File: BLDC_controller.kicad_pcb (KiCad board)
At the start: 4 copper layers, 50 x 35 mm, 95 parts, among them P2 CONN_01X06, P3 CONN_01X05, P5 CONN_01X05, Q1 PSMN2R0-30YLD, Q2 PSMN2R0-30YLD, Q3 PSMN2R0-30YLD, Q4 PSMN2R0-30YLD, Q5 PSMN2R0-30YLD, Q6 PSMN2R0-30YLD

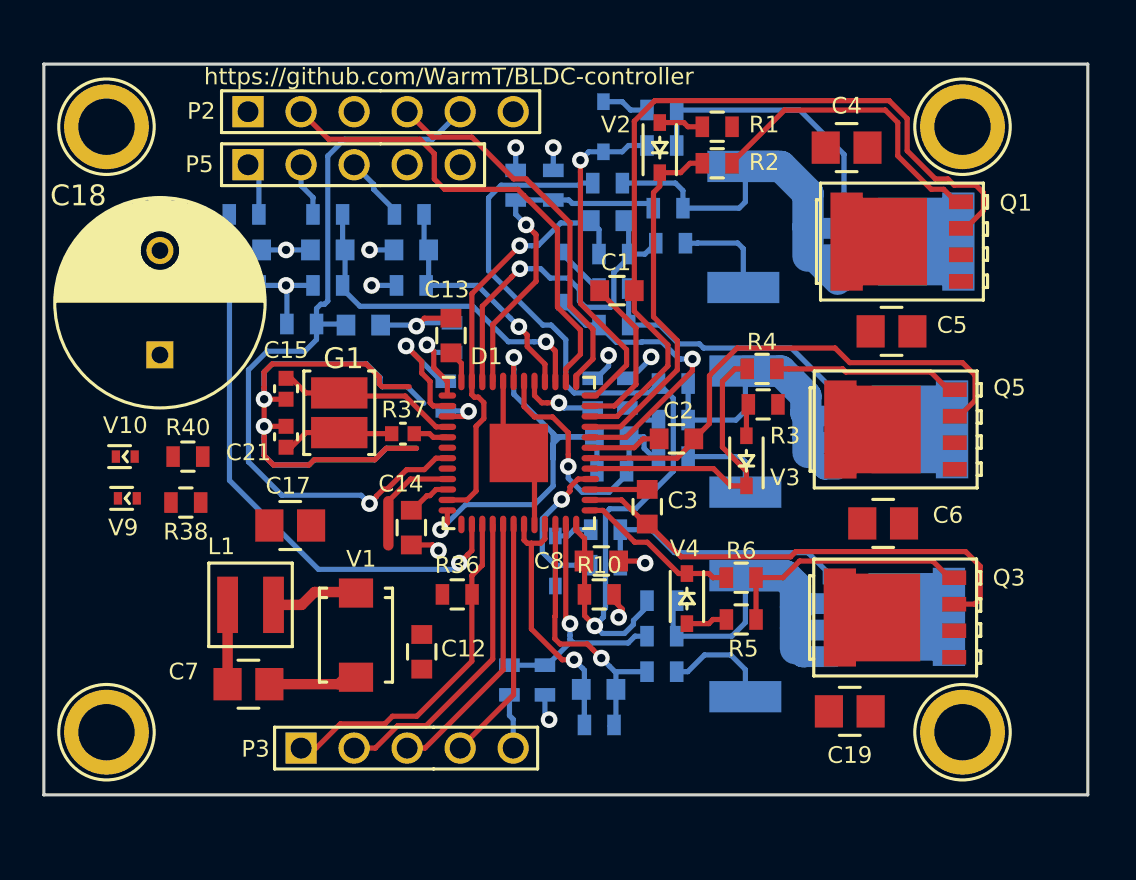
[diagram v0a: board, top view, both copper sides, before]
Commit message: Layout ready for 1st review
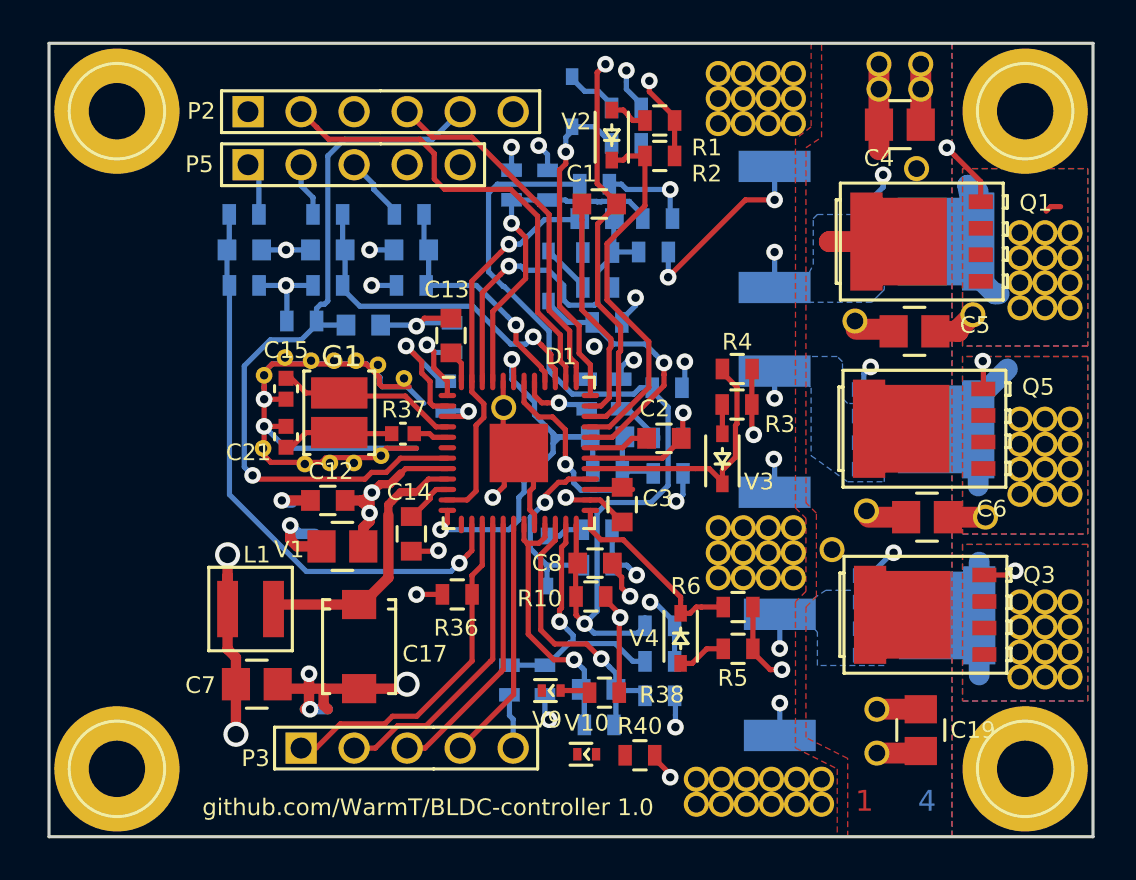
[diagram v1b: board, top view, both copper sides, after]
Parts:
- removed C18: 680u, project_footprints:C_Radial_D10_L25_P5
- added REF**: VIA-0.8mm-0.4mm, project_footprints:VIA-0.8mm-0.4mm, F.Cu at (151.2, 97.8)
- added REF**: VIA-0.8mm-0.4mm, project_footprints:VIA-0.8mm-0.4mm, F.Cu at (149.9, 93.2)
- added REF**: VIA-1.2mm-0.8mm, project_footprints:VIA-1.2mm-0.8mm, F.Cu at (166.2, 113.2)
- added REF**: VIA-0.8mm-0.4mm, project_footprints:VIA-0.8mm-0.4mm, F.Cu at (147.8, 93.2)
- added REF**: VIA-0.8mm-0.4mm, project_footprints:VIA-0.8mm-0.4mm, F.Cu at (148.9, 93.2)
- added REF**: VIA-1.2mm-0.8mm, project_footprints:VIA-1.2mm-0.8mm, F.Cu at (172.8, 102.3)
- added REF**: VIA-1.2mm-0.8mm, project_footprints:VIA-1.2mm-0.8mm, F.Cu at (180.1, 100.7)
- added REF**: VIA-1.2mm-0.8mm, project_footprints:VIA-1.2mm-0.8mm, F.Cu at (174.9, 112.0)
- added REF**: VIA-1.2mm-0.8mm, project_footprints:VIA-1.2mm-0.8mm, F.Cu at (174.9, 109.9)
- added REF**: VIA-1.2mm-0.8mm, project_footprints:VIA-1.2mm-0.8mm, F.Cu at (174.4, 100.4)
- added REF**: VIA-1.2mm-0.8mm, project_footprints:VIA-1.2mm-0.8mm, F.Cu at (173.8, 91.3)
- added REF**: VIA-1.2mm-0.8mm, project_footprints:VIA-1.2mm-0.8mm, F.Cu at (179.5, 91.0)
- added REF**: VIA-1.2mm-0.8mm, project_footprints:VIA-1.2mm-0.8mm, F.Cu at (176.8, 84.0)
- added REF**: VIA-0.8mm-0.4mm, project_footprints:VIA-0.8mm-0.4mm, F.Cu at (149.8, 98.1)
- added REF**: VIA-1.2mm-0.8mm, project_footprints:VIA-1.2mm-0.8mm, F.Cu at (177.0, 79.0)
- added REF**: VIA-1.2mm-0.8mm, project_footprints:VIA-1.2mm-0.8mm, F.Cu at (177.0, 80.2)
- added REF**: VIA-1.2mm-0.8mm, project_footprints:VIA-1.2mm-0.8mm, F.Cu at (175.0, 80.2)
- added REF**: VIA-1.2mm-0.8mm, project_footprints:VIA-1.2mm-0.8mm, F.Cu at (175.0, 79.0)
- added REF**: VIA-1.2mm-0.8mm, project_footprints:VIA-1.2mm-0.8mm, F.Cu at (170.9, 81.8)
- added REF**: VIA-1.2mm-0.8mm, project_footprints:VIA-1.2mm-0.8mm, F.Cu at (169.7, 81.8)
- added REF**: VIA-1.2mm-0.8mm, project_footprints:VIA-1.2mm-0.8mm, F.Cu at (168.5, 81.8)
- added REF**: VIA-1.2mm-0.8mm, project_footprints:VIA-1.2mm-0.8mm, F.Cu at (167.3, 81.8)
- added REF**: VIA-1.2mm-0.8mm, project_footprints:VIA-1.2mm-0.8mm, F.Cu at (170.9, 80.7)
- added REF**: VIA-1.2mm-0.8mm, project_footprints:VIA-1.2mm-0.8mm, F.Cu at (169.7, 80.7)
- added REF**: VIA-0.8mm-0.4mm, project_footprints:VIA-0.8mm-0.4mm, F.Cu at (148.7, 98.1)
- added REF**: VIA-1.2mm-0.8mm, project_footprints:VIA-1.2mm-0.8mm, F.Cu at (168.5, 80.7)
- added REF**: VIA-1.2mm-0.8mm, project_footprints:VIA-1.2mm-0.8mm, F.Cu at (167.3, 80.7)
- added REF**: VIA-1.2mm-0.8mm, project_footprints:VIA-1.2mm-0.8mm, F.Cu at (170.9, 79.5)
- added REF**: VIA-1.2mm-0.8mm, project_footprints:VIA-1.2mm-0.8mm, F.Cu at (169.7, 79.5)
- added REF**: VIA-1.2mm-0.8mm, project_footprints:VIA-1.2mm-0.8mm, F.Cu at (168.5, 79.5)
- added REF**: VIA-1.2mm-0.8mm, project_footprints:VIA-1.2mm-0.8mm, F.Cu at (169.7, 103.6)
- added REF**: VIA-1.2mm-0.8mm, project_footprints:VIA-1.2mm-0.8mm, F.Cu at (168.5, 103.6)
- added REF**: VIA-1.2mm-0.8mm, project_footprints:VIA-1.2mm-0.8mm, F.Cu at (167.3, 103.6)
- added REF**: VIA-1.2mm-0.8mm, project_footprints:VIA-1.2mm-0.8mm, F.Cu at (170.9, 103.6)
- added REF**: VIA-1.2mm-0.8mm, project_footprints:VIA-1.2mm-0.8mm, F.Cu at (169.7, 102.4)
- added REF**: VIA-0.8mm-0.4mm, project_footprints:VIA-0.8mm-0.4mm, F.Cu at (146.6, 93.1)
- added REF**: VIA-1.2mm-0.8mm, project_footprints:VIA-1.2mm-0.8mm, F.Cu at (168.5, 102.4)
- added REF**: VIA-1.2mm-0.8mm, project_footprints:VIA-1.2mm-0.8mm, F.Cu at (167.3, 102.4)
- added REF**: VIA-1.2mm-0.8mm, project_footprints:VIA-1.2mm-0.8mm, F.Cu at (170.9, 102.4)
- added REF**: VIA-1.2mm-0.8mm, project_footprints:VIA-1.2mm-0.8mm, F.Cu at (169.7, 101.2)
- added REF**: VIA-1.2mm-0.8mm, project_footprints:VIA-1.2mm-0.8mm, F.Cu at (168.5, 101.2)
- added REF**: VIA-1.2mm-0.8mm, project_footprints:VIA-1.2mm-0.8mm, F.Cu at (167.3, 101.2)
- added REF**: VIA-1.2mm-0.8mm, project_footprints:VIA-1.2mm-0.8mm, F.Cu at (170.9, 101.2)
- added REF**: VIA-1.2mm-0.8mm, project_footprints:VIA-1.2mm-0.8mm, F.Cu at (184.2, 108.4)
- added REF**: VIA-1.2mm-0.8mm, project_footprints:VIA-1.2mm-0.8mm, F.Cu at (182.9, 108.4)
- added REF**: VIA-1.2mm-0.8mm, project_footprints:VIA-1.2mm-0.8mm, F.Cu at (181.8, 108.4)
- added REF**: VIA-0.8mm-0.4mm, project_footprints:VIA-0.8mm-0.4mm, F.Cu at (147.5, 98.2)
- added REF**: VIA-1.2mm-0.8mm, project_footprints:VIA-1.2mm-0.8mm, F.Cu at (184.2, 107.2)
- added REF**: VIA-1.2mm-0.8mm, project_footprints:VIA-1.2mm-0.8mm, F.Cu at (182.9, 107.2)
- added REF**: VIA-1.2mm-0.8mm, project_footprints:VIA-1.2mm-0.8mm, F.Cu at (181.8, 107.2)
- added REF**: VIA-1.2mm-0.8mm, project_footprints:VIA-1.2mm-0.8mm, F.Cu at (184.2, 106.0)
- added REF**: VIA-1.2mm-0.8mm, project_footprints:VIA-1.2mm-0.8mm, F.Cu at (182.9, 106.0)
- added REF**: VIA-1.2mm-0.8mm, project_footprints:VIA-1.2mm-0.8mm, F.Cu at (181.8, 106.0)
- added REF**: VIA-1.2mm-0.8mm, project_footprints:VIA-1.2mm-0.8mm, F.Cu at (184.2, 104.8)
- added REF**: VIA-1.2mm-0.8mm, project_footprints:VIA-1.2mm-0.8mm, F.Cu at (182.9, 104.8)
- added REF**: VIA-1.2mm-0.8mm, project_footprints:VIA-1.2mm-0.8mm, F.Cu at (181.8, 104.8)
- added REF**: VIA-1.2mm-0.8mm, project_footprints:VIA-1.2mm-0.8mm, F.Cu at (184.2, 99.6)
- added REF**: VIA-0.8mm-0.4mm, project_footprints:VIA-0.8mm-0.4mm, F.Cu at (145.5, 97.4)
- added REF**: VIA-1.2mm-0.8mm, project_footprints:VIA-1.2mm-0.8mm, F.Cu at (182.9, 99.6)
- added REF**: VIA-1.2mm-0.8mm, project_footprints:VIA-1.2mm-0.8mm, F.Cu at (181.8, 99.6)
- added REF**: VIA-1.2mm-0.8mm, project_footprints:VIA-1.2mm-0.8mm, F.Cu at (184.2, 98.4)
- added REF**: VIA-1.2mm-0.8mm, project_footprints:VIA-1.2mm-0.8mm, F.Cu at (182.9, 98.4)
- added REF**: VIA-1.2mm-0.8mm, project_footprints:VIA-1.2mm-0.8mm, F.Cu at (181.8, 98.4)
- added REF**: VIA-1.2mm-0.8mm, project_footprints:VIA-1.2mm-0.8mm, F.Cu at (184.2, 97.2)
- added REF**: VIA-1.2mm-0.8mm, project_footprints:VIA-1.2mm-0.8mm, F.Cu at (182.9, 97.2)
- added REF**: VIA-1.2mm-0.8mm, project_footprints:VIA-1.2mm-0.8mm, F.Cu at (181.8, 97.2)
- added REF**: VIA-1.2mm-0.8mm, project_footprints:VIA-1.2mm-0.8mm, F.Cu at (184.2, 96.0)
- added REF**: VIA-1.2mm-0.8mm, project_footprints:VIA-1.2mm-0.8mm, F.Cu at (182.9, 96.0)
- added REF**: VIA-0.8mm-0.4mm, project_footprints:VIA-0.8mm-0.4mm, F.Cu at (145.6, 93.9)
- added REF**: VIA-1.2mm-0.8mm, project_footprints:VIA-1.2mm-0.8mm, F.Cu at (181.8, 96.0)
- added REF**: VIA-1.2mm-0.8mm, project_footprints:VIA-1.2mm-0.8mm, F.Cu at (184.2, 90.7)
- added REF**: VIA-1.2mm-0.8mm, project_footprints:VIA-1.2mm-0.8mm, F.Cu at (182.9, 90.7)
- added REF**: VIA-1.2mm-0.8mm, project_footprints:VIA-1.2mm-0.8mm, F.Cu at (181.8, 90.7)
- added REF**: VIA-1.2mm-0.8mm, project_footprints:VIA-1.2mm-0.8mm, F.Cu at (184.2, 89.5)
- added REF**: VIA-1.2mm-0.8mm, project_footprints:VIA-1.2mm-0.8mm, F.Cu at (182.9, 89.5)
- added REF**: VIA-1.2mm-0.8mm, project_footprints:VIA-1.2mm-0.8mm, F.Cu at (181.8, 89.5)
- added REF**: VIA-1.2mm-0.8mm, project_footprints:VIA-1.2mm-0.8mm, F.Cu at (184.2, 88.3)
- added REF**: VIA-1.2mm-0.8mm, project_footprints:VIA-1.2mm-0.8mm, F.Cu at (182.9, 88.3)
- added REF**: VIA-1.2mm-0.8mm, project_footprints:VIA-1.2mm-0.8mm, F.Cu at (181.8, 88.3)
- added REF**: VIA-0.8mm-0.4mm, project_footprints:VIA-0.8mm-0.4mm, F.Cu at (152.2, 94.1)
- added REF**: VIA-1.2mm-0.8mm, project_footprints:VIA-1.2mm-0.8mm, F.Cu at (184.2, 87.1)
- added REF**: VIA-1.2mm-0.8mm, project_footprints:VIA-1.2mm-0.8mm, F.Cu at (182.9, 87.1)
- added REF**: VIA-1.2mm-0.8mm, project_footprints:VIA-1.2mm-0.8mm, F.Cu at (181.8, 87.1)
- added REF**: VIA-1.2mm-0.8mm, project_footprints:VIA-1.2mm-0.8mm, F.Cu at (157.0, 95.5)
- added REF**: VIA-1.2mm-0.8mm, project_footprints:VIA-1.2mm-0.8mm, F.Cu at (172.2, 114.5)
- added REF**: VIA-1.2mm-0.8mm, project_footprints:VIA-1.2mm-0.8mm, F.Cu at (171.1, 114.5)
- added REF**: VIA-1.2mm-0.8mm, project_footprints:VIA-1.2mm-0.8mm, F.Cu at (169.8, 114.5)
- added REF**: VIA-1.2mm-0.8mm, project_footprints:VIA-1.2mm-0.8mm, F.Cu at (168.7, 114.5)
- added REF**: VIA-1.2mm-0.8mm, project_footprints:VIA-1.2mm-0.8mm, F.Cu at (167.4, 114.5)
- added REF**: VIA-0.8mm-0.4mm, project_footprints:VIA-0.8mm-0.4mm, F.Cu at (151.0, 93.4)
- added REF**: VIA-1.2mm-0.8mm, project_footprints:VIA-1.2mm-0.8mm, F.Cu at (166.2, 114.5)
- added REF**: VIA-1.2mm-0.8mm, project_footprints:VIA-1.2mm-0.8mm, F.Cu at (172.2, 113.2)
- added REF**: VIA-1.2mm-0.8mm, project_footprints:VIA-1.2mm-0.8mm, F.Cu at (171.1, 113.2)
- added REF**: VIA-1.2mm-0.8mm, project_footprints:VIA-1.2mm-0.8mm, F.Cu at (169.8, 113.2)
- added REF**: VIA-1.2mm-0.8mm, project_footprints:VIA-1.2mm-0.8mm, F.Cu at (168.7, 113.2)
- added REF**: VIA-1.2mm-0.8mm, project_footprints:VIA-1.2mm-0.8mm, F.Cu at (167.4, 113.2)
- added REF**: VIA-1.2mm-0.8mm, project_footprints:VIA-1.2mm-0.8mm, F.Cu at (167.3, 79.5)
- moved V10 26.3 mm to (161.0, 112.1)
- moved R40 25.9 mm to (163.6, 112.1)
- moved V9 22.3 mm to (159.3, 109.0)
- moved R38 22.0 mm to (161.8, 109.1)
- moved C12 8.53 mm to (148.6, 99.9), turned to 180 degrees
- moved C1 4.24 mm to (161.6, 85.7)
- moved C19 3.52 mm to (177.0, 110.9), turned to 270 degrees
- moved REF** 3.48 mm to (182.0, 112.8)
- moved REF** 3.09 mm to (182.0, 81.3)
- moved C4 2.78 mm to (176.0, 81.9)
- moved R2 2.77 mm to (164.5, 83.4)
- moved R1 2.77 mm to (164.5, 81.7)
- moved C17 2.69 mm to (149.3, 102.1), turned to 180 degrees
- moved R7 2.48 mm to (170.2, 108.3)
- moved V2 2.38 mm to (162.2, 82.4)
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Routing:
- net GND: track 81.5 -> 114.7 mm, vias 9 -> 20
- net +12V: track 0.00 -> 25.7 mm, vias 0 -> 3
- net /OUTW: track 23.5 -> 37.0 mm, vias 0 -> 1
- net +3V3: track 18.5 -> 30.0 mm, vias 6 -> 9
- net /OUTU: track 39.3 -> 49.9 mm, vias 0 -> 1
- net V_SENSE_P: track 17.6 -> 7.63 mm, vias 0 -> 2
- net /HSU: track 14.8 -> 24.0 mm, vias 0 -> 2
- net U_SENSE_P: track 21.1 -> 12.4 mm, vias 0 -> 2
- net /HSV: track 8.63 -> 17.2 mm, vias 0 -> 2
- net /OUTV: track 25.1 -> 33.3 mm, vias 0 -> 1
- net /LSV: track 13.1 -> 20.6 mm, vias 0 -> 2
- net W_SENSE_P: track 19.3 -> 12.2 mm, vias 0 -> 2
- net /LSU: track 12.9 -> 19.8 mm, vias 0 -> 2
- net /LSW: track 13.5 -> 20.0 mm, vias 0 -> 2
- net /HSW: track 12.2 -> 18.6 mm, vias 0 -> 2
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- added copper zone on F.Cu, net +12V
- added copper zone on In1.Cu, net +12V
- added copper zone on In2.Cu, net +12V
- added copper zone on In1.Cu, net +3V3
- added copper zone on B.Cu, net /OUTU
- added copper zone on F.Cu, net /OUTU
- added copper zone on In2.Cu, net /OUTU
- added copper zone on B.Cu, net /OUTV
- added copper zone on F.Cu, net /OUTV
- added copper zone on In2.Cu, net /OUTV
- added copper zone on B.Cu, net /OUTW
- added copper zone on F.Cu, net /OUTW
- added copper zone on In2.Cu, net /OUTW
- added copper zone on F.Cu, net GND
- added copper zone on In2.Cu, net GND
- added copper zone on B.Cu, net U_SENSE_P
- added copper zone on B.Cu, net V_SENSE_P
- added copper zone on B.Cu, net W_SENSE_P
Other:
- board size 50 x 35 mm -> 50 x 38 mm
- rule trace_min: 0.15 -> 0.25
- board text added: "1"
- board text added: "2"
- board text added: "3"
- board text added: "4"
- board text added: "github.com/WarmT/BLDC-controller 1.0"
- board text removed: "https://github.com/WarmT/BLDC-controller"
